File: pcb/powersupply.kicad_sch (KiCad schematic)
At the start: 29 parts, among them Q10 2N7002, Q9 2N7002, U10 SMAJ16A-TR, U4 TPS54302, U5 SMAJ16A-TR, U6 AMS1117-3.3, U9 CJ431

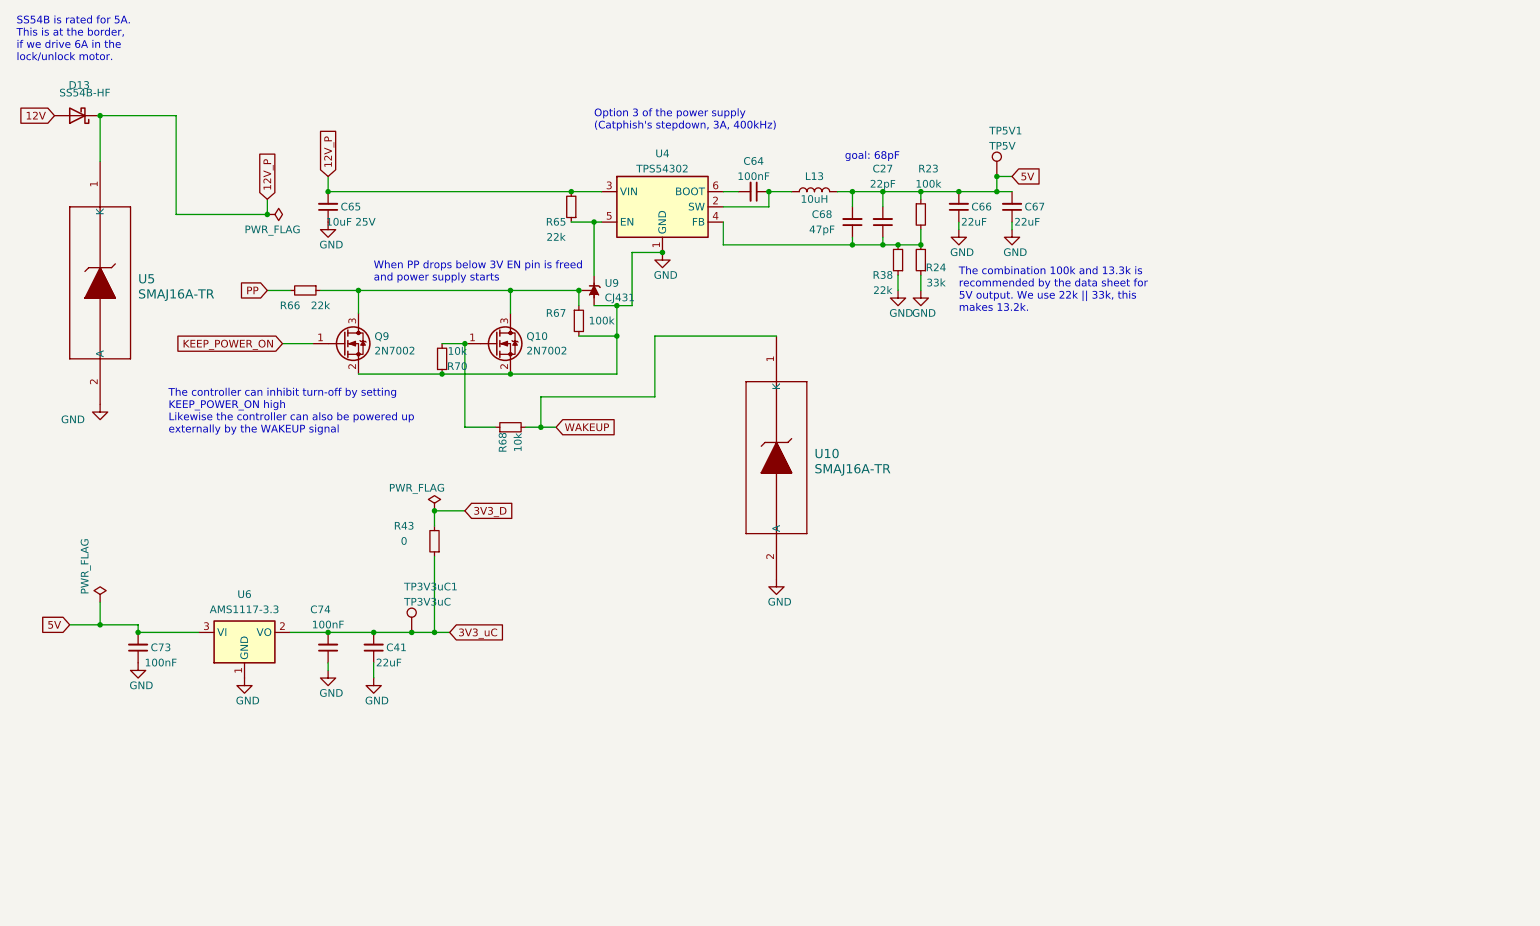
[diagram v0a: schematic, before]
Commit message: Redesigned wakeup circuit
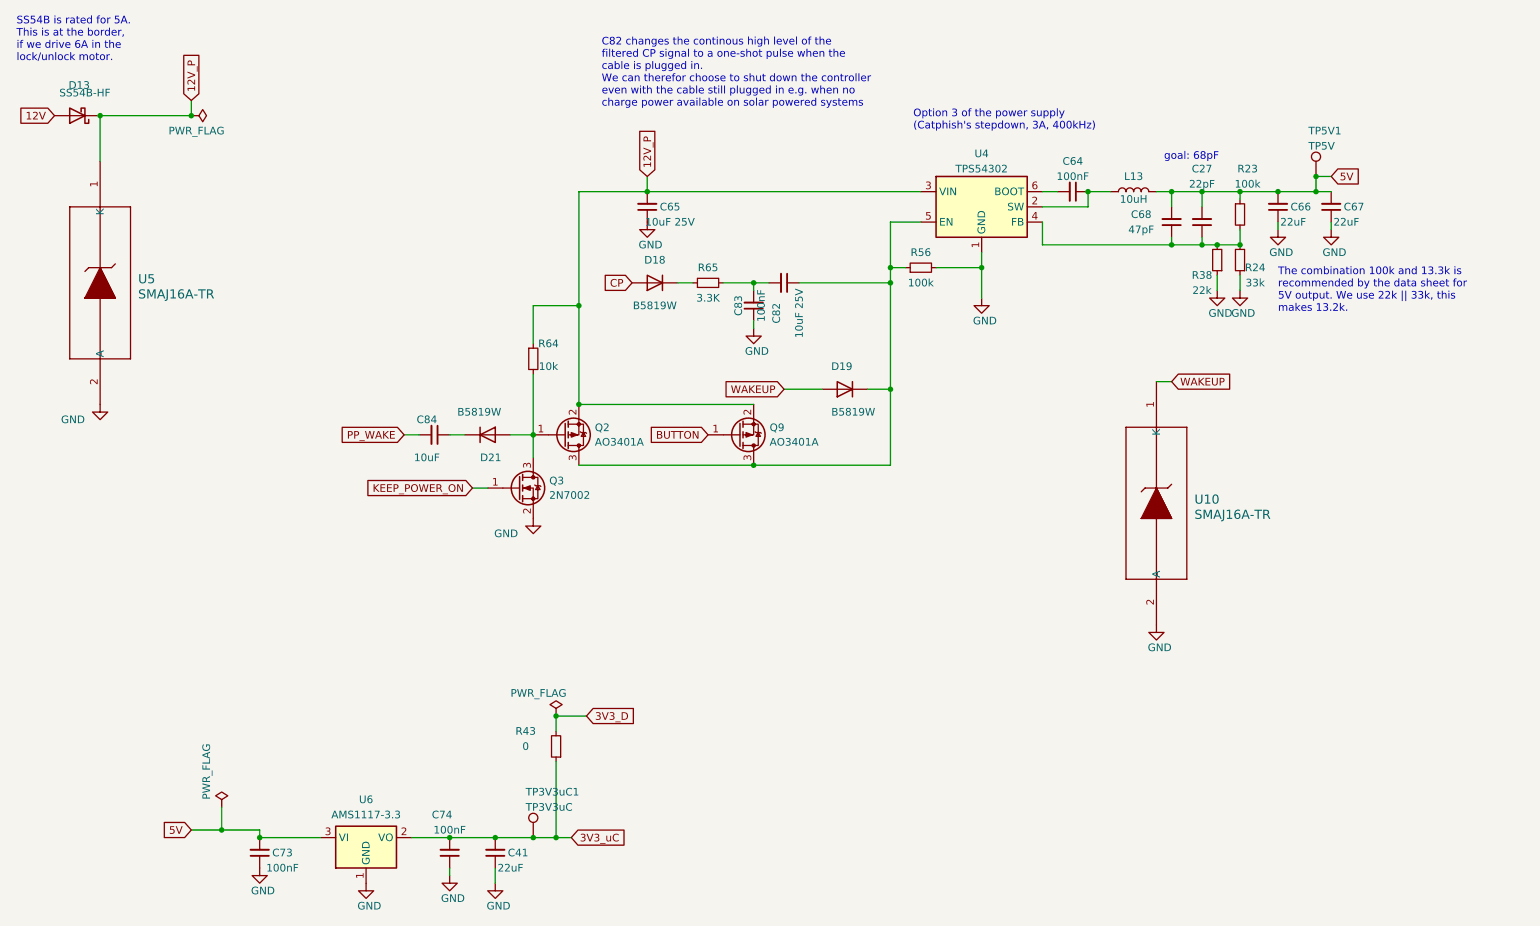
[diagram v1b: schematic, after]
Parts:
- removed Q10, Q9: 2N7002, Package_TO_SOT_SMD:SOT-23, symbol Transistor_FET:2N7002
- removed R66: 22k, Resistor_SMD:R_0805_2012Metric_Pad1.20x1.40mm_HandSolder, symbol Device:R_Small
- removed R67: 100k, Resistor_SMD:R_0805_2012Metric_Pad1.20x1.40mm_HandSolder, symbol Device:R_Small
- removed R68, R70: 10k, Resistor_SMD:R_0805_2012Metric_Pad1.20x1.40mm_HandSolder, symbol Device:R_Small
- removed U9: CJ431, Package_TO_SOT_SMD:SOT-23-3, symbol Reference_Voltage:CJ431DBZ
- added C82: 10uF 25V, Capacitor_SMD:C_0805_2012Metric_Pad1.18x1.45mm_HandSolder, symbol Device:C_Small
- added C83: 100nF, Capacitor_SMD:C_0805_2012Metric_Pad1.18x1.45mm_HandSolder, symbol Device:C_Small
- added C84: 10uF, Capacitor_SMD:C_0805_2012Metric_Pad1.18x1.45mm_HandSolder, symbol Device:C_Small
- added D18, D19, D21: B5819W, Diode_SMD:D_SOD-123, symbol Diode:1N4148W
- added Q2, Q9: AO3401A, Package_TO_SOT_SMD:SOT-23, symbol Transistor_FET:AO3401A
- added Q3: 2N7002, Package_TO_SOT_SMD:SOT-23, symbol Transistor_FET:2N7002
- added R56: 100k, Resistor_SMD:R_0805_2012Metric_Pad1.20x1.40mm_HandSolder, symbol Device:R_Small
- added R64: 10k, Resistor_SMD:R_0805_2012Metric_Pad1.20x1.40mm_HandSolder, symbol Device:R_Small
- R65: value 22k -> 3.3K; LCSC C17560 -> C26010; LINK https://jlcpcb.com/partdetail/18248-0805W8F2202T5E/C17560 -> https://jlcpcb.com/partdetail/26753-0805W8F3301T5E/C26010
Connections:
- net 12V_P: now also Q2.2 (S), Q9.2 (S), R64.1; no longer R65.2
- net GND: now also C83.1, Q3.2 (S), R56.2
- net KEEP_POWER_ON: now also Q3.1 (G)
- net WAKEUP: now also D19.2 (A)
- net at U4.5 (EN): now also C82.1, D19.1 (K), Q2.3 (D), Q9.3 (D), R56.1; no longer R65.1
- new net: D21.2 (A), Q2.1 (G), Q3.3 (D), R64.2
- new net: C82.2, C83.2, R65.2
- new net: C84.1, D21.1 (K)
- new net: D18.1 (K), R65.1
- new net BUTTON: Q9.1 (G)
- new net CP: D18.2 (A)
- new net PP_WAKE: C84.2
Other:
- note added: "C82 changes the continous high level of the filtered CP signal to a one-shot pulse when the cable is plugged in. We can therefor choose to shut down the controller even with the cable still plugged in e.g. when no charge power available on solar powered systems"
- note removed: "The controller can inhibit turn-off by setting KEEP_POWER_ON high Likewise the controller can also be powered up externally by the WAKEUP signal"
- note removed: "When PP drops below 3V EN pin is freed and power supply starts"
- moved on the sheet: C27, C41, C64, C65, C66, C67, C68, C73, C74, L13, R23, R24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

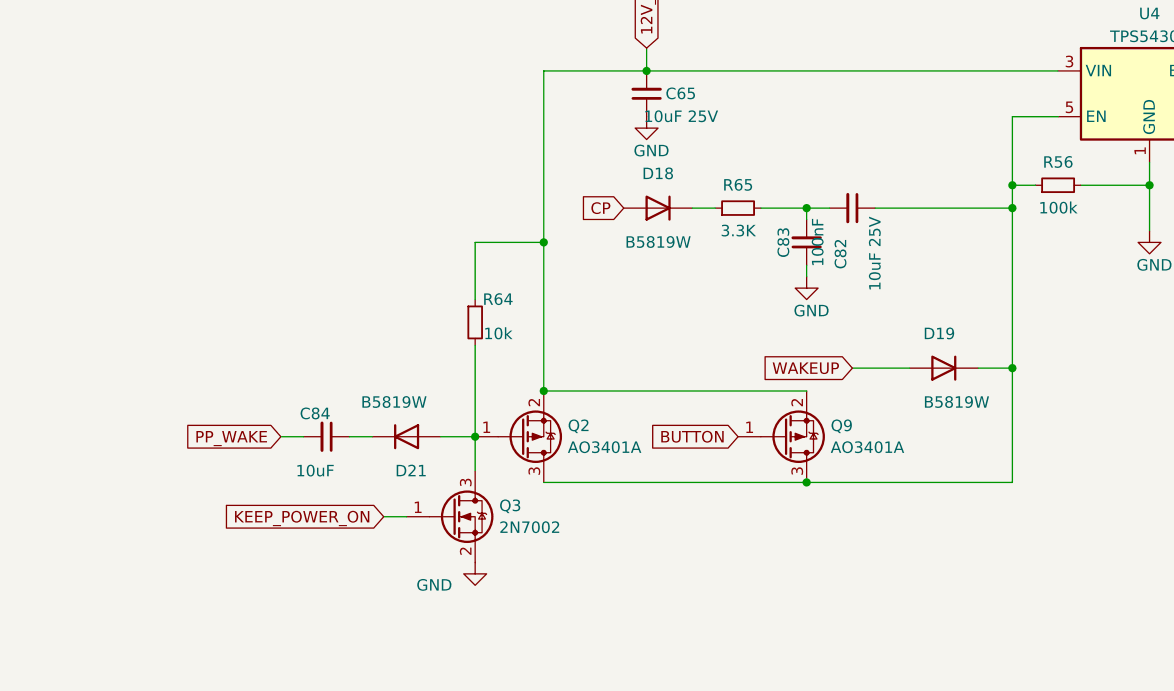
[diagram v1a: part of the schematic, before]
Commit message: Added 1M discharge resistor for CP enable Removed momentary turn-on resitor for PP enable because always charged by uC voltage divider
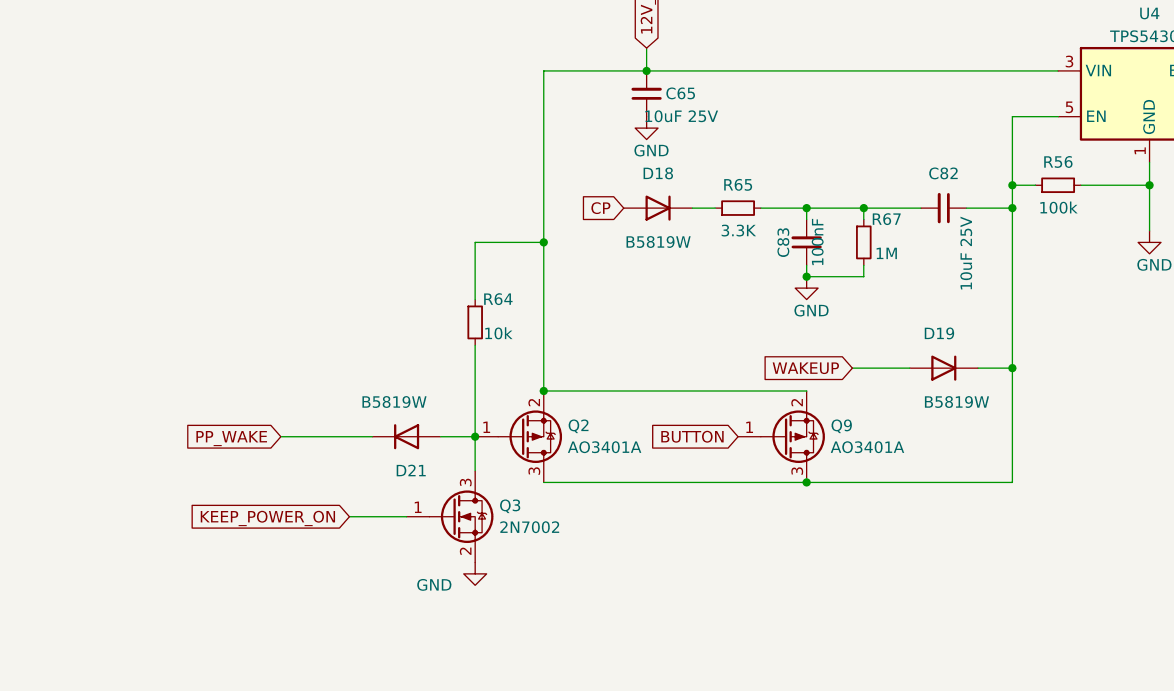
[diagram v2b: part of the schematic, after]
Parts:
- removed C84: 10uF, Capacitor_SMD:C_0805_2012Metric_Pad1.18x1.45mm_HandSolder, symbol Device:C_Small
- added R67: 1M, Resistor_SMD:R_0805_2012Metric_Pad1.20x1.40mm_HandSolder, symbol Device:R_Small
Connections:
- net GND: now also R67.2
- net PP_WAKE: now also D21.1 (K)
- net at C82.2, C83.2, R65.2: now also R67.1
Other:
- moved on the sheet: C82
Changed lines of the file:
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@@
   (junction (at 227.33 53.34) (diameter 0) (color 0 0 0 0)
   )
+  (junction (at 152.4 59.69) (diameter 0) (color 0 0 0 0)
+  )
+  (junction (at 146.05 67.31) (diameter 0) (color 0 0 0 0)
+  )
   (junction (at 168.91 57.15) (diameter 0) (color 0 0 0 0)
   )
@@
     (stroke (width 0) (type default))
   )
-  (wire (pts (xy 95.25 85.09) (xy 97.79 85.09))
-    (stroke (width 0) (type default))
-  )
   (wire (pts (xy 168.91 59.69) (xy 168.91 77.47))
     (stroke (width 0) (type default))
@@
     (stroke (width 0) (type default))
   )
+  (wire (pts (xy 152.4 67.31) (xy 146.05 67.31))
+    (stroke (width 0) (type default))
+  )
   (wire (pts (xy 151.13 77.47) (xy 157.48 77.47))
     (stroke (width 0) (type default))
@@
     (stroke (width 0) (type default))
   )
+  (wire (pts (xy 152.4 59.69) (xy 158.75 59.69))
+    (stroke (width 0) (type default))
+  )
+  (wire (pts (xy 152.4 59.69) (xy 152.4 60.96))
+    (stroke (width 0) (type default))
+  )
   (wire (pts (xy 233.68 49.53) (xy 233.68 50.8))
     (stroke (width 0) (type default))
@@
     (stroke (width 0) (type default))
   )
-  (wire (pts (xy 87.63 85.09) (xy 90.17 85.09))
+  (wire (pts (xy 87.63 85.09) (xy 97.79 85.09))
     (stroke (width 0) (type default))
   )
@@
     (stroke (width 0) (type default))
   )
+  (wire (pts (xy 152.4 66.04) (xy 152.4 67.31))
+    (stroke (width 0) (type default))
+  )
   (wire (pts (xy 168.91 57.15) (xy 168.91 59.69))
     (stroke (width 0) (type default))
   )
-  (wire (pts (xy 153.67 59.69) (xy 168.91 59.69))
+  (wire (pts (xy 163.83 59.69) (xy 168.91 59.69))
     (stroke (width 0) (type default))
   )
@@
     (stroke (width 0) (type default))
   )
-  (wire (pts (xy 146.05 59.69) (xy 148.59 59.69))
-    (stroke (width 0) (type default))
-  )
-  (wire (pts (xy 99.06 93.98) (xy 101.6 93.98))
+  (wire (pts (xy 146.05 59.69) (xy 152.4 59.69))
+    (stroke (width 0) (type default))
+  )
+  (wire (pts (xy 95.25 93.98) (xy 101.6 93.98))
     (stroke (width 0) (type default))
   )
@@
     )
   )
-  (global_label "KEEP_POWER_ON" (shape input) (at 99.06 93.98 180) (fields_autoplaced)
+  (global_label "KEEP_POWER_ON" (shape input) (at 95.25 93.98 180) (fields_autoplaced)
     (effects (font (size 1.27 1.27)) (justify right))
-    (property "Intersheetrefs" "${INTERSHEET_REFS}" (at 80.1697 93.98 0)
+    (property "Intersheetrefs" "${INTERSHEET_REFS}" (at 76.3597 93.98 0)
       (effects (font (size 1.27 1.27)) (justify right) hide)
     )
@@
     )
   )
-  (symbol (lib_id "Device:C_Small") (at 151.13 59.69 270) (unit 1)
-    (in_bom yes) (on_board yes) (dnp no)
-    (property "Reference" "C82" (at 149.86 64.77 0)
-      (effects (font (size 1.27 1.27)))
-    )
-    (property "Value" "10uF 25V" (at 153.67 64.77 0)
-      (effects (font (size 1.27 1.27)))
-    )
-    (property "Footprint" "Capacitor_SMD:C_0805_2012Metric_Pad1.18x1.45mm_HandSolder" (at 151.13 59.69 0)
-      (effects (font (size 1.27 1.27)) hide)
-    )
-    (property "Datasheet" "https://datasheet.lcsc.com/lcsc/1811110921_Samsung-Electro-Mechanics-CL10A106MA8NRNC_C96446.pdf" (at 151.13 59.69 0)
-      (effects (font (size 1.27 1.27)) hide)
-    )
-    (property "LCSC" "C15850" (at 151.13 59.69 0)
-      (effects (font (size 1.27 1.27)) hide)
-    )
-    (property "LINK" "https://jlcpcb.com/partdetail/16532-CL21A106KAYNNNE/C15850" (at 151.13 59.69 0)
+  (symbol (lib_id "Device:C_Small") (at 161.29 59.69 270) (unit 1)
+    (in_bom yes) (on_board yes) (dnp no)
+    (property "Reference" "C82" (at 161.29 55.88 90)
+      (effects (font (size 1.27 1.27)))
+    )
+    (property "Value" "10uF 25V" (at 163.83 64.77 0)
+      (effects (font (size 1.27 1.27)))
+    )
+    (property "Footprint" "Capacitor_SMD:C_0805_2012Metric_Pad1.18x1.45mm_HandSolder" (at 161.29 59.69 0)
+      (effects (font (size 1.27 1.27)) hide)
+    )
+    (property "Datasheet" "https://datasheet.lcsc.com/lcsc/1811110921_Samsung-Electro-Mechanics-CL10A106MA8NRNC_C96446.pdf" (at 161.29 59.69 0)
+      (effects (font (size 1.27 1.27)) hide)
+    )
+    (property "LCSC" "C15850" (at 161.29 59.69 0)
+      (effects (font (size 1.27 1.27)) hide)
+    )
+    (property "LINK" "https://jlcpcb.com/partdetail/16532-CL21A106KAYNNNE/C15850" (at 161.29 59.69 0)
       (effects (font (size 1.27 1.27)) hide)
     )
@@
     )
   )
+  (symbol (lib_id "Device:R_Small") (at 152.4 63.5 0) (unit 1)
+    (in_bom yes) (on_board yes) (dnp no)
+    (property "Reference" "R67" (at 154.94 60.96 0)
+      (effects (font (size 1.27 1.27)))
+    )
+    (property "Value" "1M" (at 154.94 64.77 0)
+      (effects (font (size 1.27 1.27)))
+    )
+    (property "Footprint" "Resistor_SMD:R_0805_2012Metric_Pad1.20x1.40mm_HandSolder" (at 152.4 63.5 0)
+      (effects (font (size 1.27 1.27)) hide)
+    )
+    (property "Datasheet" "~" (at 152.4 63.5 0)
+      (effects (font (size 1.27 1.27)) hide)
+    )
+    (property "LCSC" "C22935" (at 152.4 63.5 0)
+      (effects (font (size 1.27 1.27)) hide)
+    )
+    (property "LINK" "https://jlcpcb.com/partdetail/23662-0603WAF1004T5E/C22935" (at 152.4 63.5 0)
+      (effects (font (size 1.27 1.27)) hide)
+    )
+    (pin "1")
+    (pin "2")
+    (instances
+      (project "qca7000"
+        (path "/e63e39d7-6ac0-4ffd-8aa3-1841a4541b55/81db238c-e53f-4d52-98ea-36a1df697651"
+          (reference "R67") (unit 1)
+        )
+      )
+    )
+  )
   (symbol (lib_id "power:GND") (at 227.33 60.96 0) (unit 1)
     (in_bom yes) (on_board yes) (dnp no)
@@
         )
       )
-    )
-  )
-  (symbol (lib_id "Device:C_Small") (at 92.71 85.09 270) (unit 1)
-    (in_bom yes) (on_board yes) (dnp no)
-    (property "Reference" "C84" (at 91.44 82.55 90)
-      (effects (font (size 1.27 1.27)))
-    )
-    (property "Value" "10uF" (at 91.44 88.9 90)
-      (effects (font (size 1.27 1.27)))
-    )
-    (property "Footprint" "Capacitor_SMD:C_0805_2012Metric_Pad1.18x1.45mm_HandSolder" (at 92.71 85.09 0)
-      (effects (font (size 1.27 1.27)) hide)
-    )
-    (property "Datasheet" "https://datasheet.lcsc.com/lcsc/1811110921_Samsung-Electro-Mechanics-CL10A106MA8NRNC_C96446.pdf" (at 92.71 85.09 0)
-      (effects (font (size 1.27 1.27)) hide)
-    )
-    (property "LCSC" "C15850" (at 92.71 85.09 0)
-      (effects (font (size 1.27 1.27)) hide)
-    )
-    (property "LINK" "https://jlcpcb.com/partdetail/16532-CL21A106KAYNNNE/C15850" (at 92.71 85.09 0)
-      (effects (font (size 1.27 1.27)) hide)
-    )
-    (pin "1")
-    (pin "2")
-    (instances
-      (project "qca7000"
-        (path "/e63e39d7-6ac0-4ffd-8aa3-1841a4541b55/81db238c-e53f-4d52-98ea-36a1df697651"
-          (reference "C84") (unit 1)
-        )
-      )

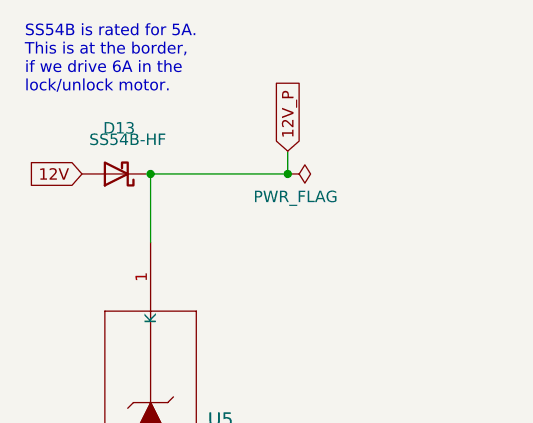
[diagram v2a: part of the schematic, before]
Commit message: BOM optimization
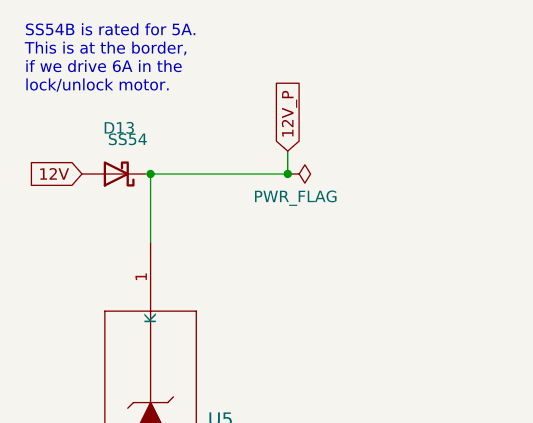
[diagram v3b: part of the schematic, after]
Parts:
- D13: value SS54B-HF -> SS54; LCSC C3014033 -> C22452; LINK https://jlcpcb.com/partdetail/Fosan-SS54B/C3014033 -> https://jlcpcb.com/partdetail/Mdd-SS54/C22452
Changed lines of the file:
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@@
       (effects (font (size 1.27 1.27)))
     )
-    (property "Value" "SS54B-HF" (at 34.29 27.94 0)
+    (property "Value" "SS54" (at 34.29 27.94 0)
       (effects (font (size 1.27 1.27)))
     )
@@
       (effects (font (size 1.27 1.27)) hide)
     )
-    (property "Datasheet" "https://www.mouser.de/datasheet/2/80/20190806170503-2505092.pdf" (at 33.02 31.75 0)
+    (property "Datasheet" "~" (at 33.02 31.75 0)
       (effects (font (size 1.27 1.27)) hide)
     )
-    (property "LCSC" "C3014033" (at 33.02 31.75 0)
+    (property "LCSC" "C22452" (at 33.02 31.75 0)
       (effects (font (size 1.27 1.27)) hide)
     )
-    (property "LINK" "https://jlcpcb.com/partdetail/Fosan-SS54B/C3014033" (at 33.02 31.75 0)
+    (property "LINK" "https://jlcpcb.com/partdetail/Mdd-SS54/C22452" (at 33.02 31.75 0)
       (effects (font (size 1.27 1.27)) hide)
     )
